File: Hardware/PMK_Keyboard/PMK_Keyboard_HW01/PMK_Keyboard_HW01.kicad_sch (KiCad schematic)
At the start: 0 parts

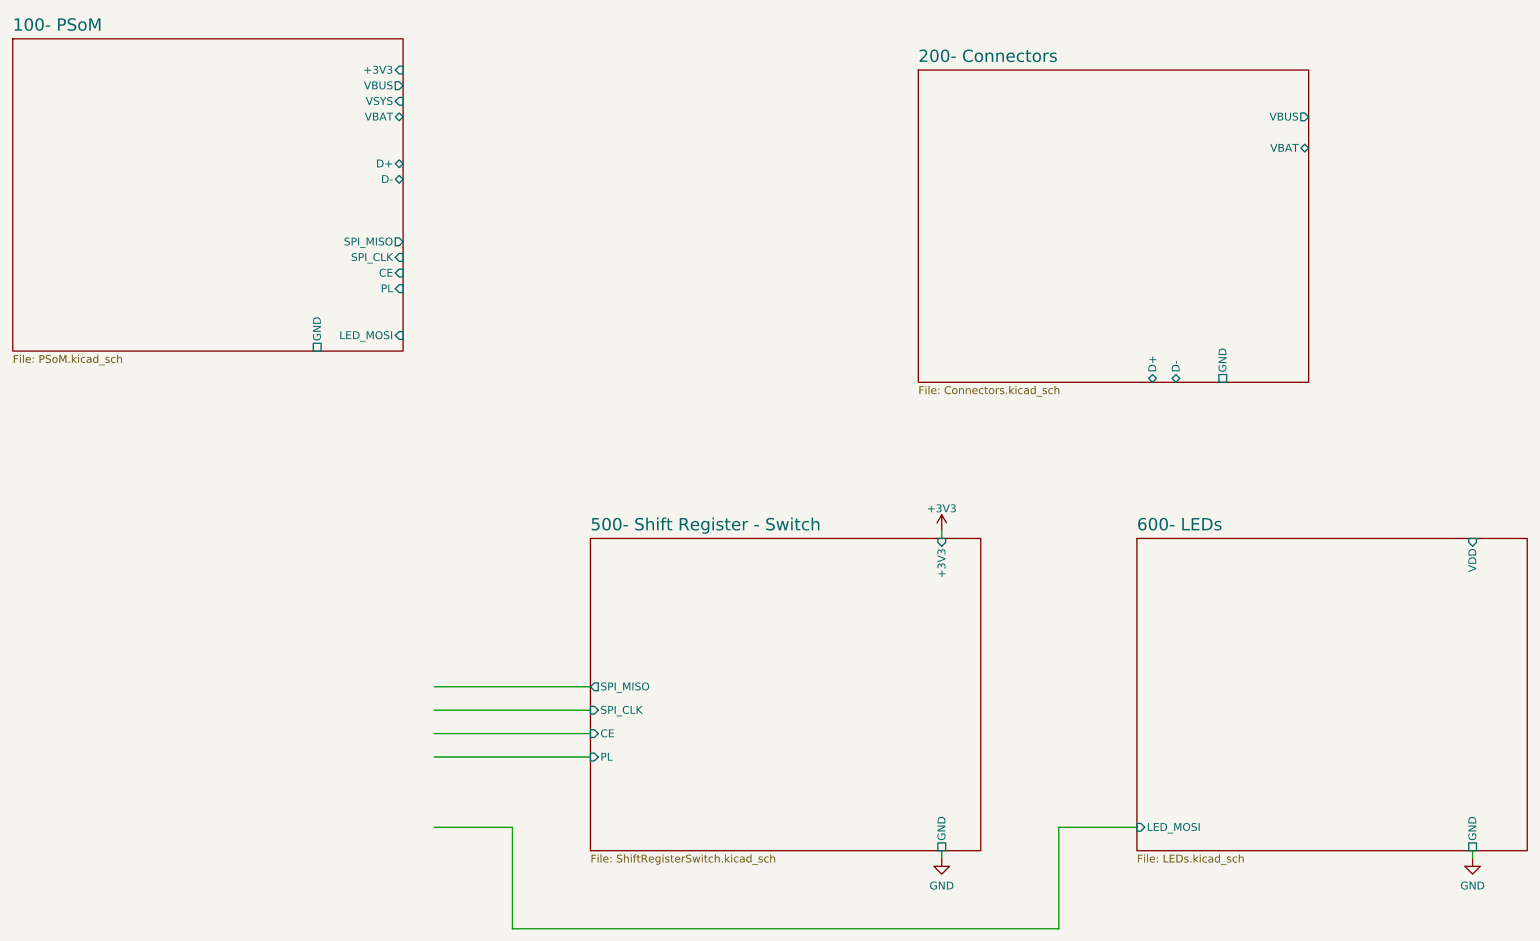
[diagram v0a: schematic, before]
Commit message: Started routing
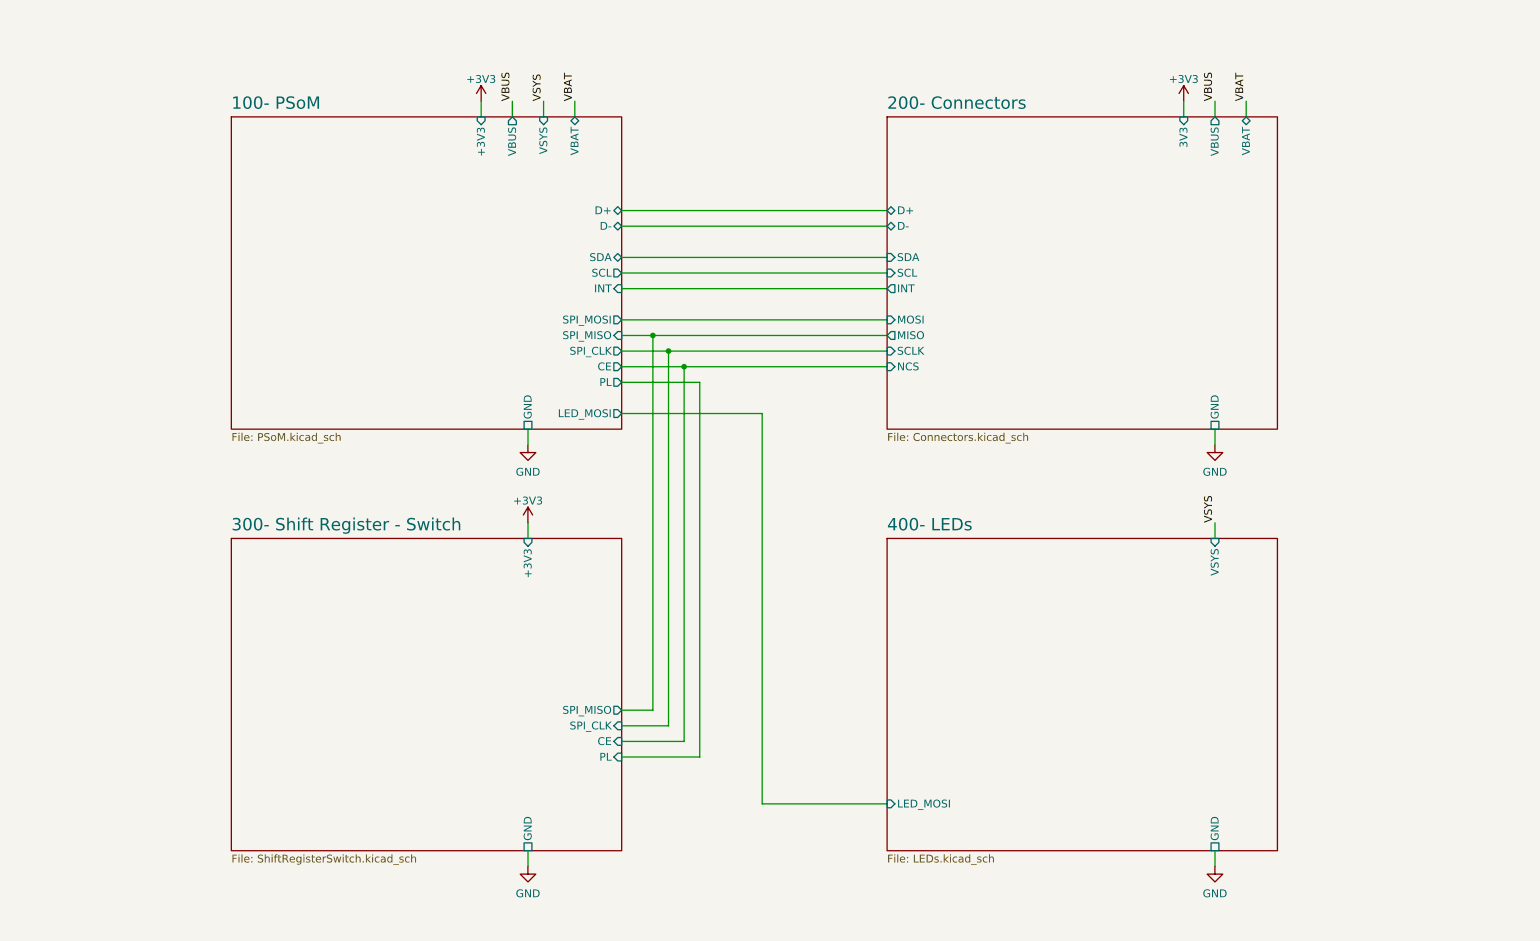
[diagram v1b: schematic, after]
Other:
- sheet 500- Shift Register - Switch renamed 300- Shift Register - Switch
- sheet 600- LEDs renamed 400- LEDs
- sheet 100- PSoM ports: added INT, SCL, SDA, SPI_MOSI; removed none
- sheet 200- Connectors ports: added 3V3, INT, MISO, MOSI, NCS, SCL, SCLK, SDA; removed none
- sheet 400- LEDs ports: added VSYS; removed VDD
